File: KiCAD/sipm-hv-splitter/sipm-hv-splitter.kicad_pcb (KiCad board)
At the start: 6 copper layers, 63.5 x 33 mm, 133 parts, among them J1 Conn_02x18_Odd_Even, J2 Conn_02x17_Odd_Even, J3 -OMIT-, Q1 BSS138, Q2 BSS138, Q3 BSS138, U1 ATmega328-M, U10 OPA810xDCK, U11 OPA810xDCK, U12 OPA810xDCK, U13 OPA810xDCK, U14 TPS7A25, U16 TPS7A25, U2 INA201, U3 LM51581, U4 LT3014xS5, U5 AD5270, U6 OPA810xDCK, U7 OPA810xDCK, U8 OPA810xDCK, U9 OPA810xDCK

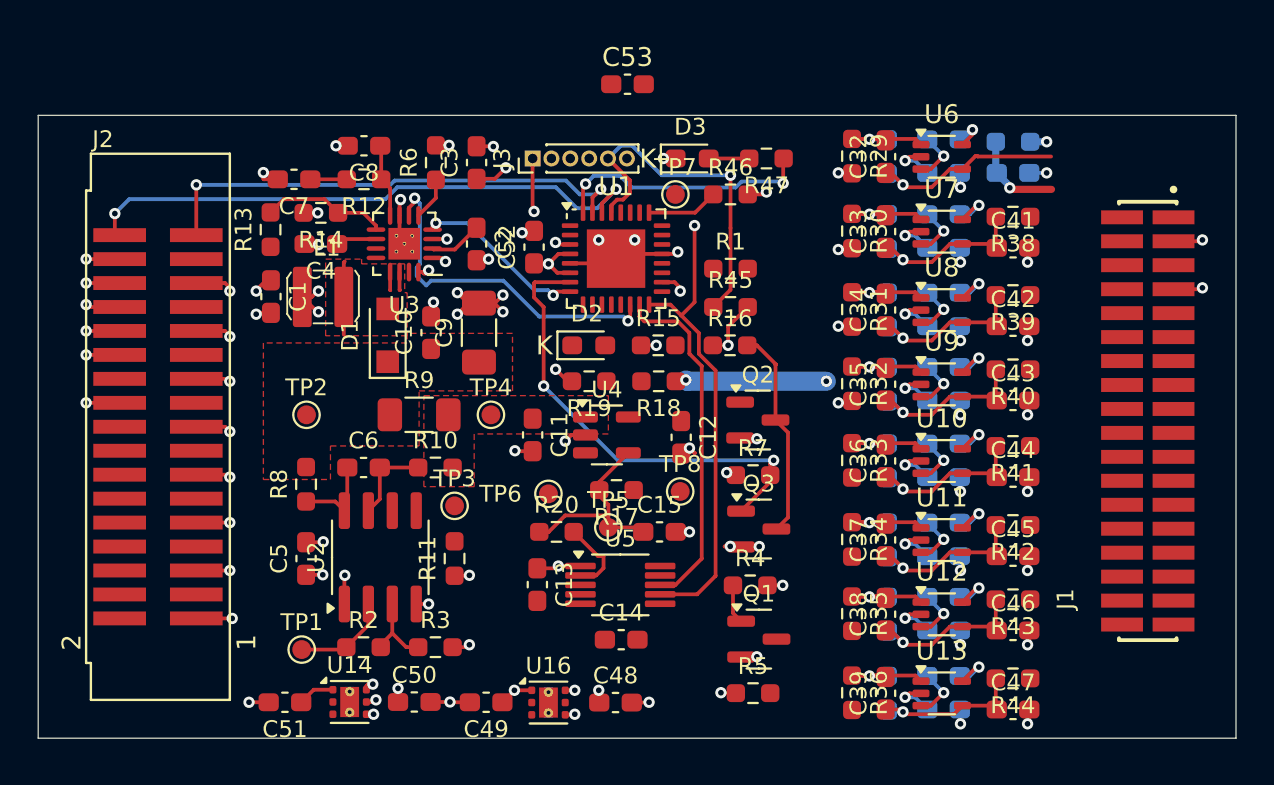
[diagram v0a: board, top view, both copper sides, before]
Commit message: routing
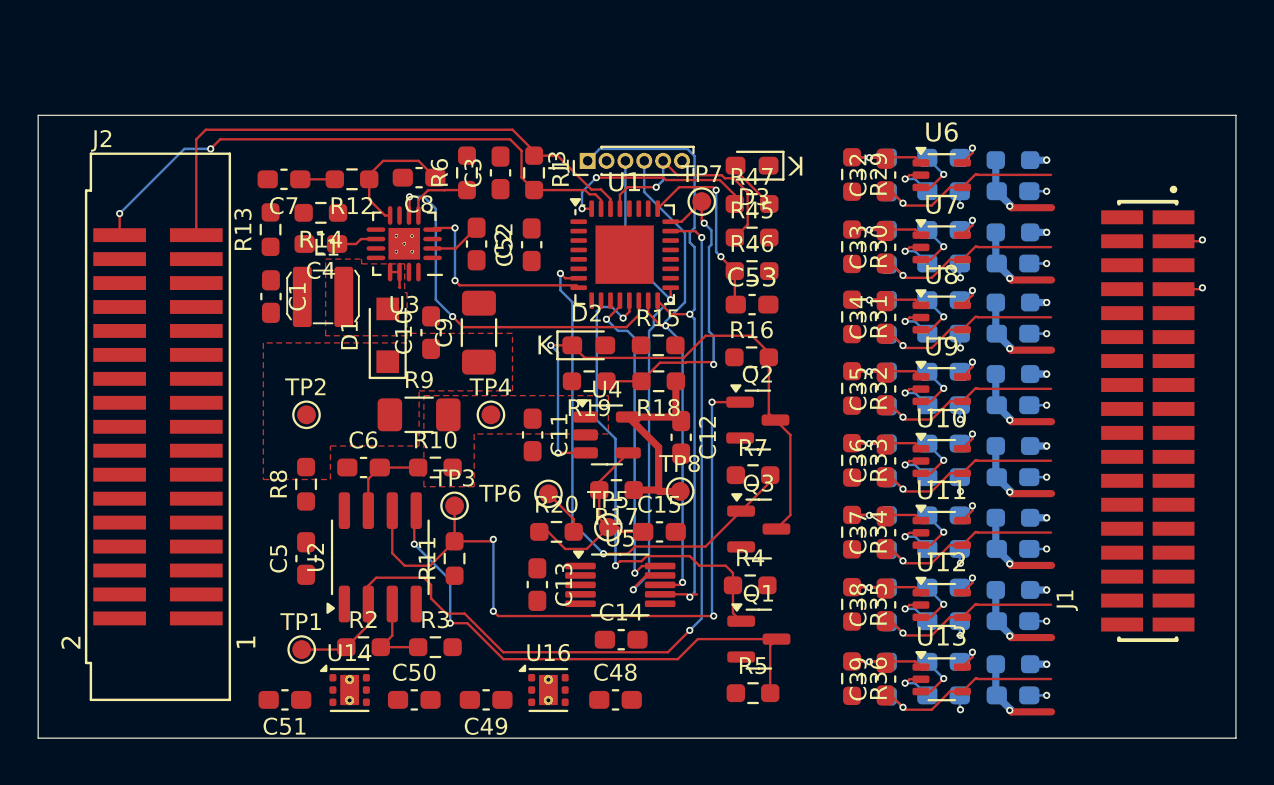
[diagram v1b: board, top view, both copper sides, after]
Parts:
- C41, C42, C43, C44, C45, C46, C47, R38, R39, R40, R41, R42, R43, R44: moved to B.Cu
- moved C53 13.4 mm to (88.6, 60.8)
- moved R1 11.6 mm to (77.1, 53.8), turned to -90 degrees
- moved R46 4.22 mm to (88.6, 59.1)
- moved R45 3.86 mm to (88.6, 57.3)
- moved C8 3.37 mm to (71.0, 54.1)
- moved D3 3.20 mm to (88.6, 53.5), turned to 180 degrees
- moved J3 2.92 mm to (79.9, 53.2)
- moved R47 2.53 mm to (88.6, 55.5), turned to 0 degrees
- moved R6 1.74 mm to (73.5, 53.8)
- moved TP7 1.45 mm to (86.0, 55.4)
- moved C3 1.38 mm to (75.3, 53.8)
- moved R16 1.31 mm to (88.6, 63.6)
- moved C24 0.97 mm to (98.8, 54.8)
- moved C40 0.97 mm to (102.5, 54.8)
- moved C16 0.97 mm to (98.8, 53.0)
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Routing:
- net /SIG_7: track 45.2 -> 0.00 mm, vias 2 -> 0
- net /ADC_IMON: track 5.19 -> 49.8 mm, vias 0 -> 2
- net /SIG_6: track 43.7 -> 0.00 mm, vias 2 -> 0
- net /SIG_5: track 43.4 -> 0.00 mm, vias 2 -> 0
- net GND: track 81.6 -> 38.6 mm, vias 65 -> 26
- net /SIG_4: track 42.4 -> 0.00 mm, vias 2 -> 0
- net Net-(Q2-G): track 0.00 -> 38.9 mm, vias 0 -> 4
- net Net-(Q1-D): track 0.00 -> 28.3 mm, vias 0 -> 2
- net /SCK: track 0.00 -> 27.0 mm, vias 0 -> 2
- net +12V: track 24.3 -> 0.00 mm, vias 19 -> 0
- net /VR_RESET: track 2.08 -> 26.2 mm, vias 0 -> 2
- net /BOOST/SHDN: track 11.2 -> 30.2 mm, vias 0 -> 2
- net +3.3V: track 18.6 -> 0.00 mm, vias 12 -> 0
- net /ADC_VMON: track 0.00 -> 17.3 mm, vias 0 -> 2
- net /~{SYNC}: track 0.00 -> 17.2 mm, vias 0 -> 2
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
